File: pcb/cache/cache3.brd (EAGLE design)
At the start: 87.6 x 86 mm, 14 parts

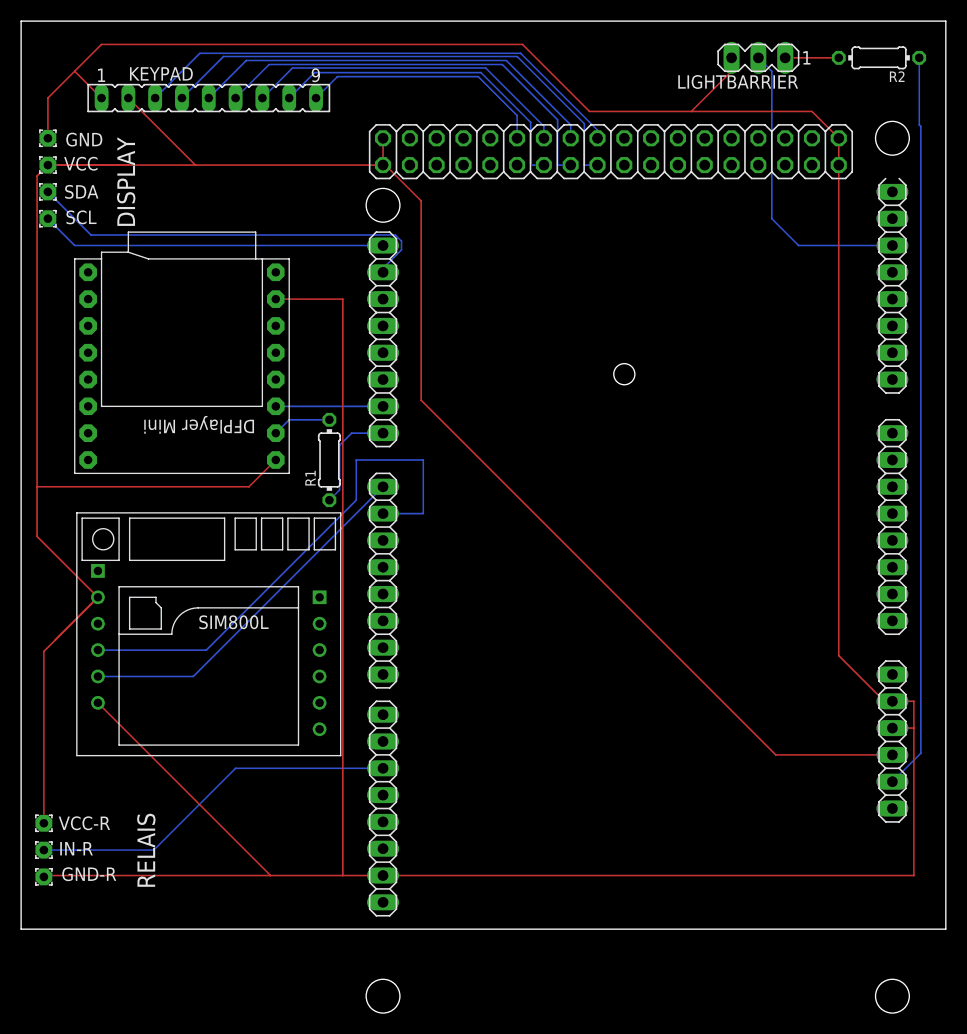
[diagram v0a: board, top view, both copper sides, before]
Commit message: updated pcb
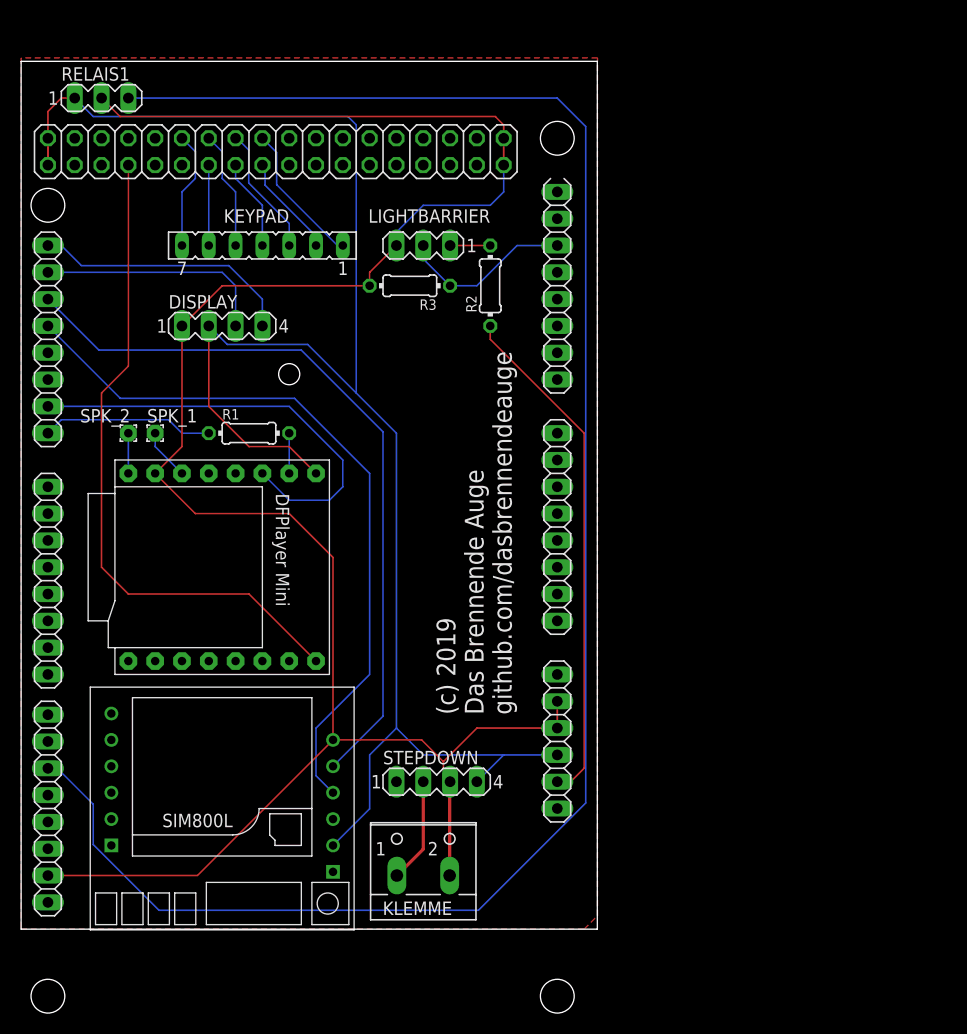
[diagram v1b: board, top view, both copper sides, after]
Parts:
- removed GND, GND-R, IN-R, SCL, SDA, VCC, VCC-R: (no value), wirepad:1,6/0,8
- added DISPLAY, STEPDOWN: (no value), con-lstb:MA04-1
- added KLEMME: (no value), con-wago-500:W237-102
- added R3: (no value), rcl:0204/7
- added RELAIS1: (no value), con-lstb:MA03-1
- added SPK_1, SPK_2: (no value), wirepad:1,6/0,8
- KEYPAD: device con-lsta:FE09 -> con-lsta:FE07
- moved R2 42.7 mm to (44.5, 61.0), turned to 90 degrees
- moved LIGHTBARRIER 36.4 mm to (38.1, 64.8)
- moved IC1 31.8 mm to (53.3, -21.6)
- moved U$1 19.4 mm to (19.1, 34.3), turned to 270 degrees
- moved U$2 16.6 mm to (19.1, 11.4), turned to 180 degrees
- moved KEYPAD 14.9 mm to (22.9, 64.8), turned to 180 degrees
- moved R1 8.03 mm to (21.6, 47.0), turned to 0 degrees
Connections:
- new net N$17: SPK_2.1, U$1.SPK2
- new net N$18: SPK_1.1, U$1.SPK1
- new net N$19: IC1.53, U$1.BUSY
- new net N$21: KLEMME.1, STEPDOWN.2
- net +5V: now also DISPLAY.2, RELAIS1.1, STEPDOWN.4; no longer KEYPAD.2, VCC-R.1, VCC.1
- net GND: now also DISPLAY.1, KLEMME.2, R3.2, RELAIS1.2, STEPDOWN.3; no longer GND-R.1, GND.1, KEYPAD.1
- net IN-B: now also R3.1
- net N$1: now also IC1.25; no longer IC1.31
- net N$10: now also KEYPAD.3; no longer KEYPAD.5
- net N$11: now also KEYPAD.2; no longer KEYPAD.4
- net N$12: now also KEYPAD.1; no longer KEYPAD.3
- net N$2: now also IC1.26; no longer IC1.32
- net N$3: now also RELAIS1.3; no longer IN-R.1
- net N$4: now also DISPLAY.3; no longer SDA.1
- net N$5: now also DISPLAY.4; no longer SCL.1
- net N$6: now also KEYPAD.7; no longer KEYPAD.9
- net N$7: now also KEYPAD.6; no longer KEYPAD.8
- net N$8: now also KEYPAD.5; no longer KEYPAD.7
- net N$9: now also KEYPAD.4; no longer KEYPAD.6
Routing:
- net N$3: track 35.3 -> 171.5 mm
- net GND: track 337.8 -> 204.6 mm
- net N$19: track 0.00 -> 63.2 mm
- net +5V: track 230.4 -> 167.6 mm
- net N$11: track 47.6 -> 9.72 mm
- net N$1: track 34.5 -> 70.6 mm
- net N$12: track 47.4 -> 13.6 mm
- net N$14: track 10.2 -> 41.8 mm
- net N$9: track 39.5 -> 8.67 mm
- net N$10: track 39.6 -> 12.3 mm
- net N$7: track 31.1 -> 7.62 mm
- net N$16: track 69.8 -> 48.7 mm
- net N$8: track 31.3 -> 11.2 mm
- net N$2: track 49.4 -> 69.3 mm
- net N$4: track 39.1 -> 22.1 mm
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- added copper zone on layer 1, net GND
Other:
- board size 87.6 x 86 mm -> 54.6 x 82.2 mm
- board text added: "(c) 2019 Das Brennende Auge github.com/dasbrennendeauge"
- board text removed: "DISPLAY"
- board text removed: "RELAIS"
